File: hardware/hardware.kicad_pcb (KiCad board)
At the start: 2 copper layers, 14.6 x 8 mm, 25 parts, among them J1 USB_B_Micro, J2 Conn_Coaxial, Q1 BSS138, Q2 BSS138, U1 ESP32-WROOM-32, U2 AMS1117-3.3, U4 CH340C, U5 RFM95W-868S2

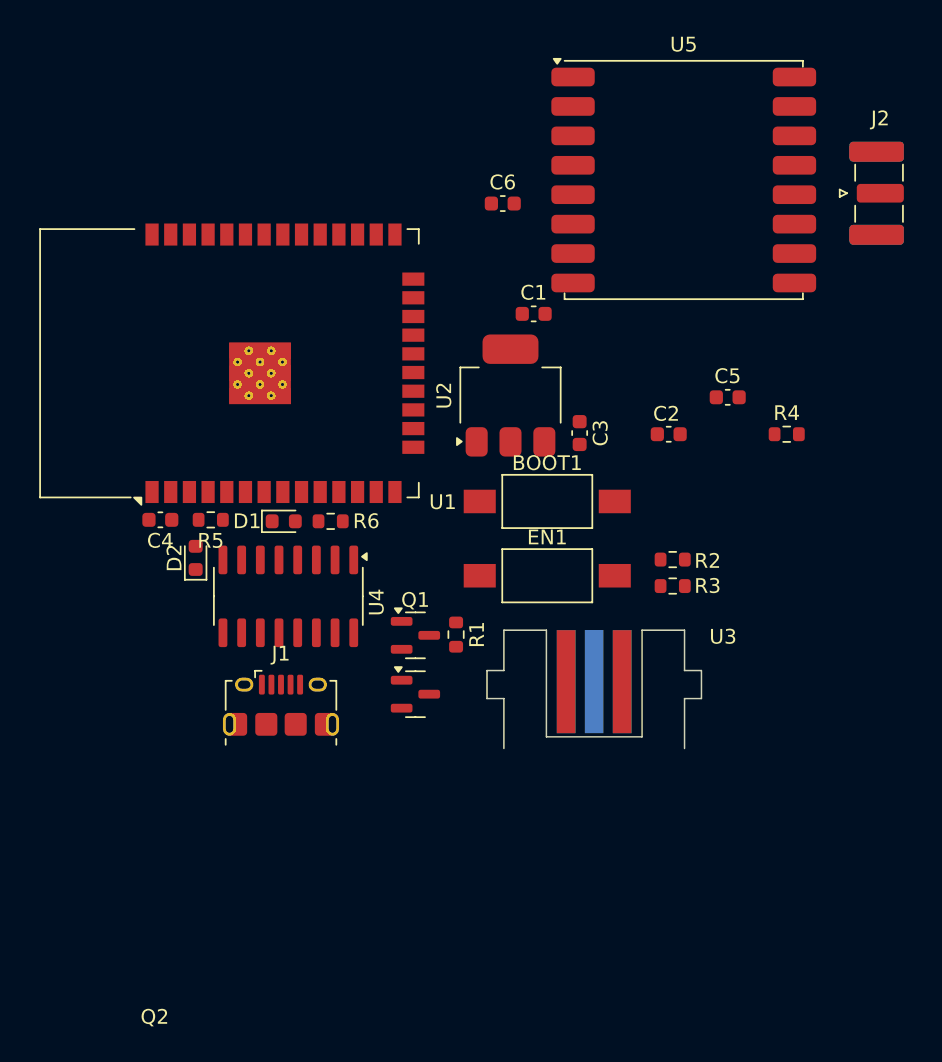
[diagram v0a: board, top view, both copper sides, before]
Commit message: lora wiring + pcb wiring
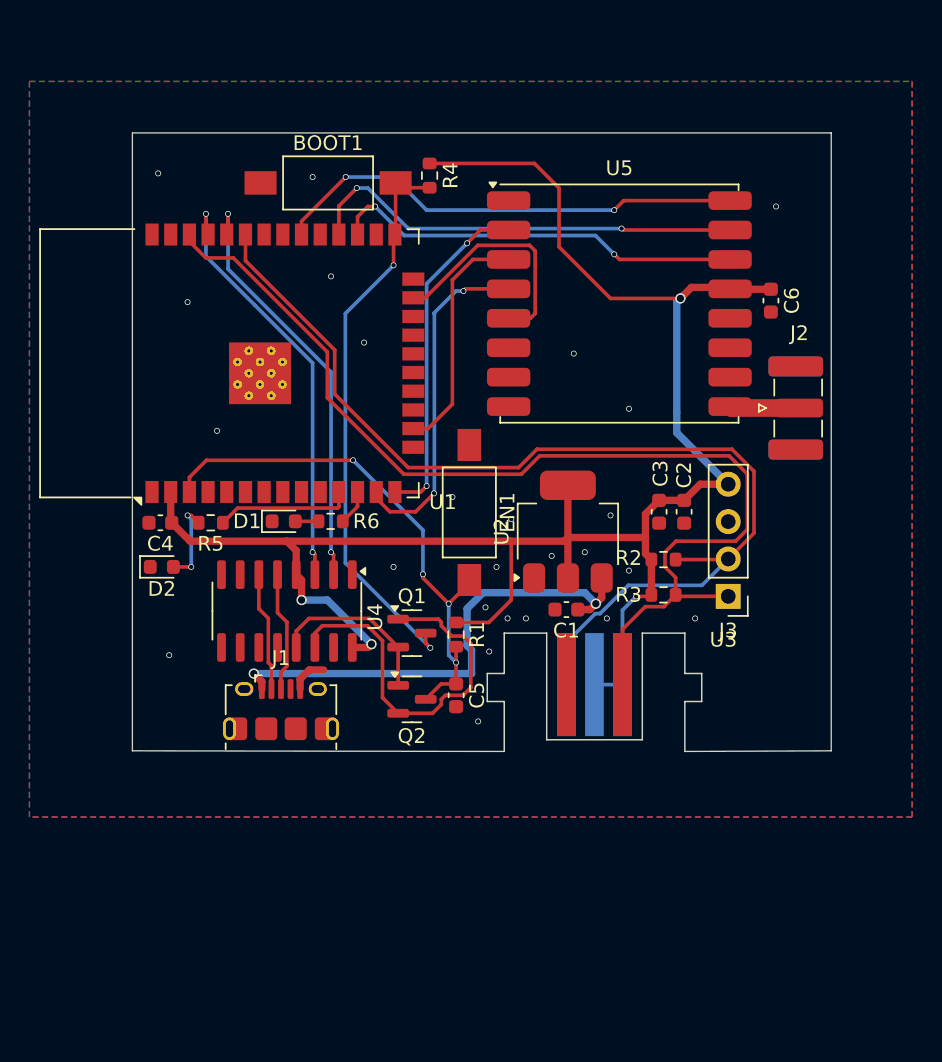
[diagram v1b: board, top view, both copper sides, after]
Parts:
- added J3: Conn_01x04, Connector_PinHeader_2.54mm:PinHeader_1x04_P2.54mm_Vertical, F.Cu at (112.5, 90.0)
- moved R4 30.0 mm to (92.2, 61.4), turned to -90 degrees
- moved C5 27.4 mm to (94.0, 96.7), turned to -90 degrees
- moved BOOT1 26.3 mm to (85.3, 61.9), turned to 180 degrees
- moved C1 20.2 mm to (101.5, 90.9), turned to 180 degrees
- moved C6 19.4 mm to (115.4, 69.9), turned to -90 degrees
- moved J2 15.6 mm to (117.3, 77.2)
- moved U2 10.0 mm to (101.6, 85.6)
- moved U5 9.47 mm to (105.1, 70.1)
- moved C3 7.60 mm to (107.8, 84.2)
- moved EN1 6.82 mm to (94.9, 84.3), turned to -90 degrees
- moved C2 5.37 mm to (109.5, 84.2), turned to -90 degrees
- moved Q1 4.36 mm to (91.0, 97.0)
- moved Q2 4.16 mm to (91.0, 92.5)
- moved D2 2.38 mm to (74.0, 88.0), turned to 0 degrees
- moved U4 1.00 mm to (82.5, 91.0)
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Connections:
- R5 pad 1: Net-(U1-IO12) -> Net-(U1-IO26)
- R6 pad 1: Net-(U1-IO13) -> Net-(U1-IO27)
- U1 pad 11: unconnected-(U1-IO26-Pad11) -> Net-(U1-IO26)
- U1 pad 12: unconnected-(U1-IO27-Pad12) -> Net-(U1-IO27)
- U1 pad 13: unconnected-(U1-IO14-Pad13) -> SCLK
- U1 pad 14: Net-(U1-IO12) -> MISO
- U1 pad 16: Net-(U1-IO13) -> MOSI
- U1 pad 23: unconnected-(U1-IO15-Pad23) -> SS
- U1 pad 27: unconnected-(U1-IO16-Pad27) -> DIO0
- U1 pad 28: unconnected-(U1-IO17-Pad28) -> DIO1
- U1 pad 30: unconnected-(U1-IO18-Pad30) -> DIO2
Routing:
- net +3V3: track 0.00 -> 126.8 mm, vias 0 -> 4
- net SCL: track 0.00 -> 73.0 mm
- net SDA: track 0.00 -> 71.6 mm
- net ESP32_IO0: track 0.00 -> 39.0 mm, vias 0 -> 2
- net ESP32_EN: track 0.00 -> 36.5 mm, vias 0 -> 4
- net +5V: track 0.00 -> 33.4 mm, vias 0 -> 2
- net DIO2: track 0.00 -> 32.5 mm, vias 0 -> 2
- net DIO1: track 0.00 -> 30.2 mm, vias 0 -> 2
- net RX-PROG: track 0.00 -> 29.1 mm, vias 0 -> 2
- net TX-PROG: track 0.00 -> 28.9 mm, vias 0 -> 2
- net DIO0: track 0.00 -> 28.3 mm, vias 0 -> 2
- net Net-(Q1-S): track 0.00 -> 26.2 mm
- net SCLK: track 0.00 -> 23.3 mm, vias 0 -> 2
- net MISO: track 0.00 -> 23.2 mm, vias 0 -> 2
- net MOSI: track 0.00 -> 16.2 mm
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- added copper zone on B.Cu, net GND
- added copper zone on F.Cu, net GND
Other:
- board size 14.6 x 8 mm -> 47.5 x 42 mm
